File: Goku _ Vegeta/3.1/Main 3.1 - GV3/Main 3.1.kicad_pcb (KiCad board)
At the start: 2 copper layers, 206 x 197.4 mm, 74 parts, among them J1 Battery Buzzer, J10 Motor 4, J11 LEFT HEADERS, J12 RIGHT HEADERS, J13 MID HEADERS, J14 UART, J15 I2C, J16 4S Battery, J17 Power Switch, J18 Batt Bal, J19 5V PI, J20 ESC PWR, J21 Line, J23 ESC PWM, J3 BACKUP 3V3, J5 SPI, J6 Solenoid, J7 Motor 1, J8 Motor 2, J9 Motor 3, Q1 BSC040N10NS5, Q2 Q_Photo_NPN, U13 Adafruit_BNO055_STEMMA_QT, U15 Bluetooth_Module_(HC-05), U16 Bluetooth_Module_(HC-06), U4 TB67H420FTG Dual/Single Motor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, U5 TB67H420FTG Dual/Single Motor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, U6 TB67H420FTG Dual/Single Motor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, U7 TB67H420FTG Dual/Single Motor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, U8 DEV-16771, U9 Arduino Compatible DC-DC Boos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

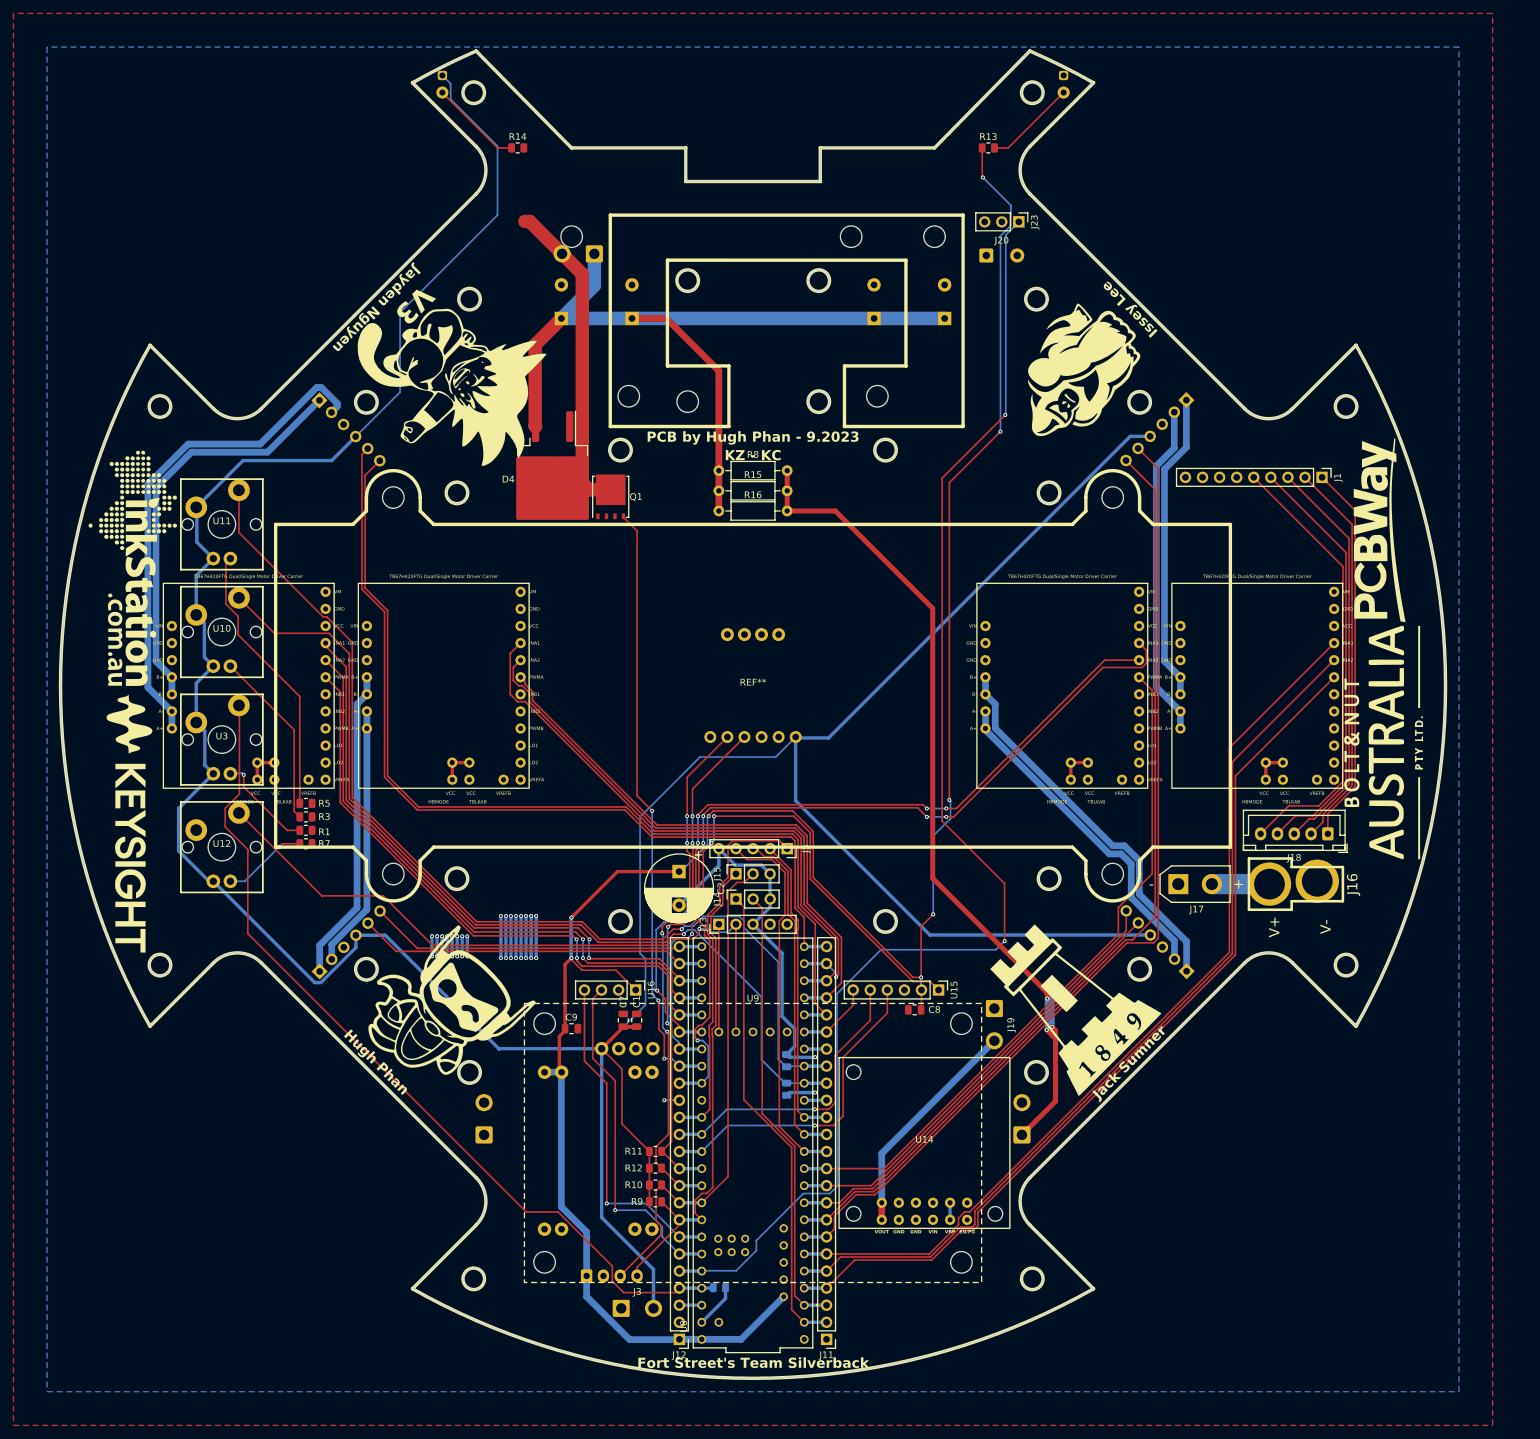
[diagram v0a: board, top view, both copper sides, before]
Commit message: main 3.1 fixup
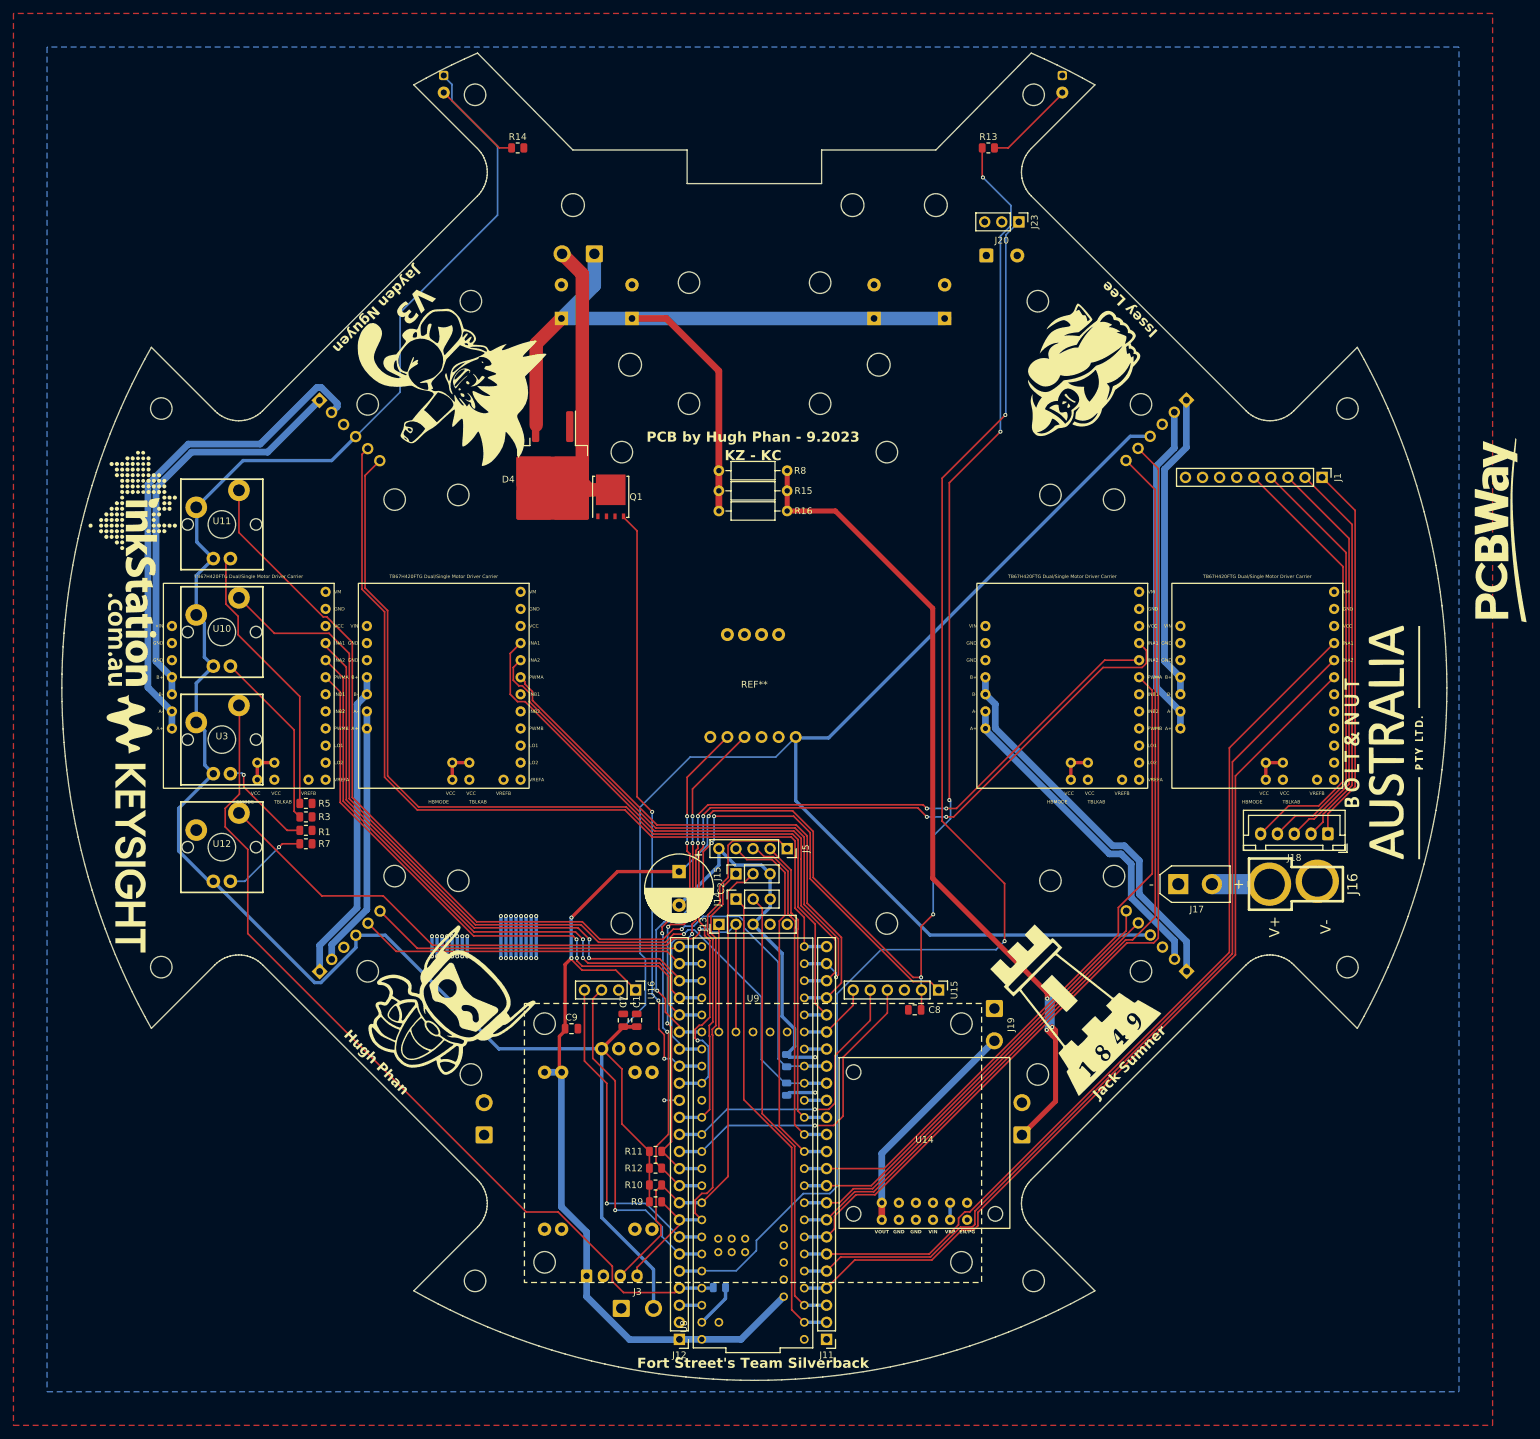
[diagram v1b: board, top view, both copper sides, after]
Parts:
- moved G*** 18.0 mm to (261.2, 127.0)
- moved REF** 0.36 mm to (150.2, 150.3)
- moved D1 0.20 mm to (196.0, 59.2)
- moved Q2 0.20 mm to (104.0, 59.2)
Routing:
- net Net-(D4-K): track 48.9 -> 41.3 mm
- net +3V3: track 518.0 -> 518.9 mm
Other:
- outline, holes or cut-outs redrawn
